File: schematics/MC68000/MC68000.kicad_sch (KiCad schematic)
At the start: 0 parts

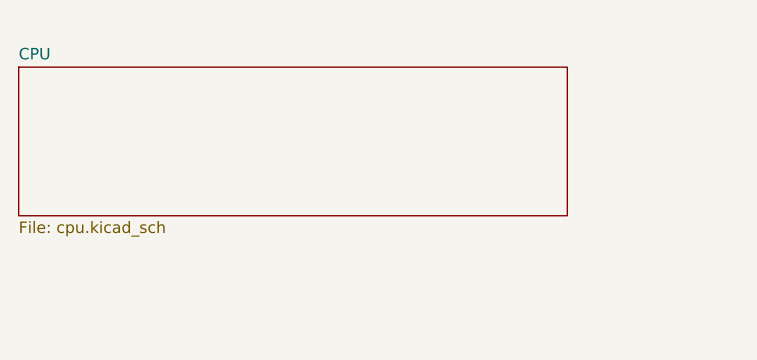
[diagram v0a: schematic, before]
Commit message: first commit
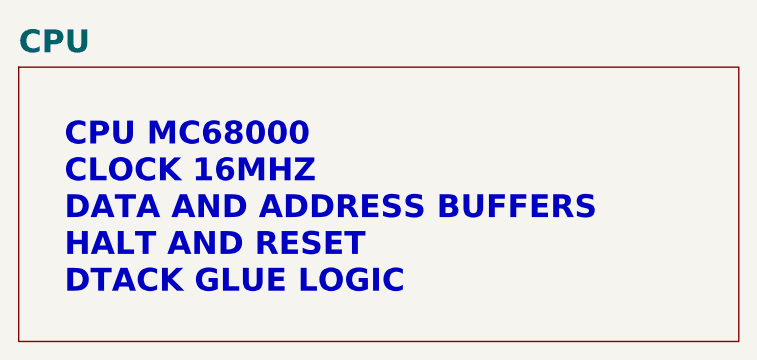
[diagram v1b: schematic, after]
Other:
- note added: "CPU MC68000 CLOCK 16MHZ DATA AND ADDRESS BUFFERS HALT AND RESET DTACK GLUE LOGIC"
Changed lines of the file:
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@@
 (kicad_sch (version 20230121) (generator eeschema)
   (paper "A3")
-  (sheet (at 31.75 31.75) (size 60.96 16.51) (fields_autoplaced)
+  (text "CPU MC68000 \nCLOCK 16MHZ\nDATA AND ADDRESS BUFFERS\nHALT AND RESET\nDTACK GLUE LOGIC\n"
+    (at 36.83 57.15 0)
+    (effects (font (size 2.54 2.54) (thickness 0.254) bold) (justify left bottom))
+  )
+  (sheet (at 31.75 31.75) (size 80.01 30.48) (fields_autoplaced)
     (stroke (width 0.1524) (type solid))
     (fill (color 0 0 0 0.0000))
-    (property "Sheetname" "CPU" (at 31.75 31.0384 0)
-      (effects (font (size 1.27 1.27)) (justify left bottom))
+    (property "Sheetname" "CPU" (at 31.75 30.4034 0) (show_name)
+      (effects (font (size 2.54 2.54) bold) (justify left bottom))
     )
-    (property "Sheetfile" "cpu.kicad_sch" (at 31.75 48.8446 0)
-      (effects (font (size 1.27 1.27)) (justify left top))
+    (property "Sheetfile" "cpu.kicad_sch" (at 31.75 62.8146 0)
+      (effects (font (size 1.27 1.27)) (justify left top) hide)
     )
     (instances
